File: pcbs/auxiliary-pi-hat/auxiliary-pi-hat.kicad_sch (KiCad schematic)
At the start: 18 parts, among them J1 Conn_01x02, J2 Raspberry Pi - Hat Template -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, J3 Conn_01x03, J4 Conn_01x03, J5 Conn_01x03, J6 Conn_01x03, J7 Conn_01x03, J8 Conn_01x04, J9 Conn_01x05, SW1 SW_Push, SW2 SW_Push, U1 YAAJ_WeAct_BlackPill_Part_Like

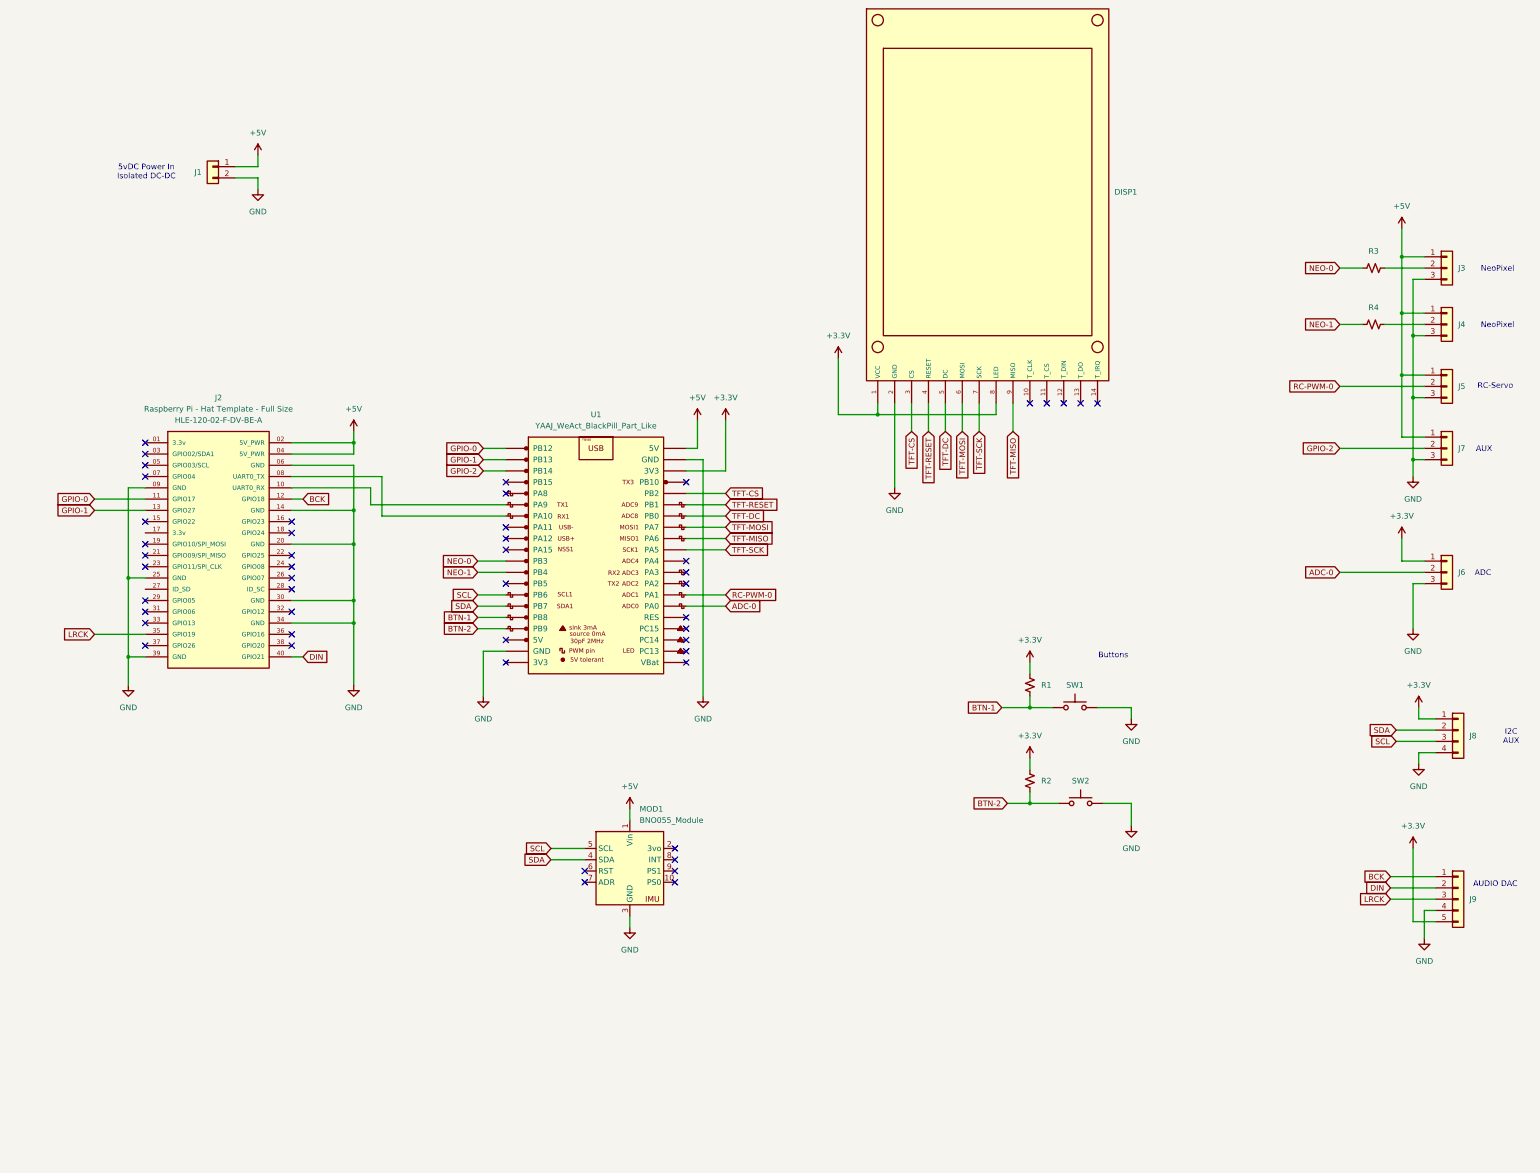
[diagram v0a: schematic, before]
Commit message: aux pcb update
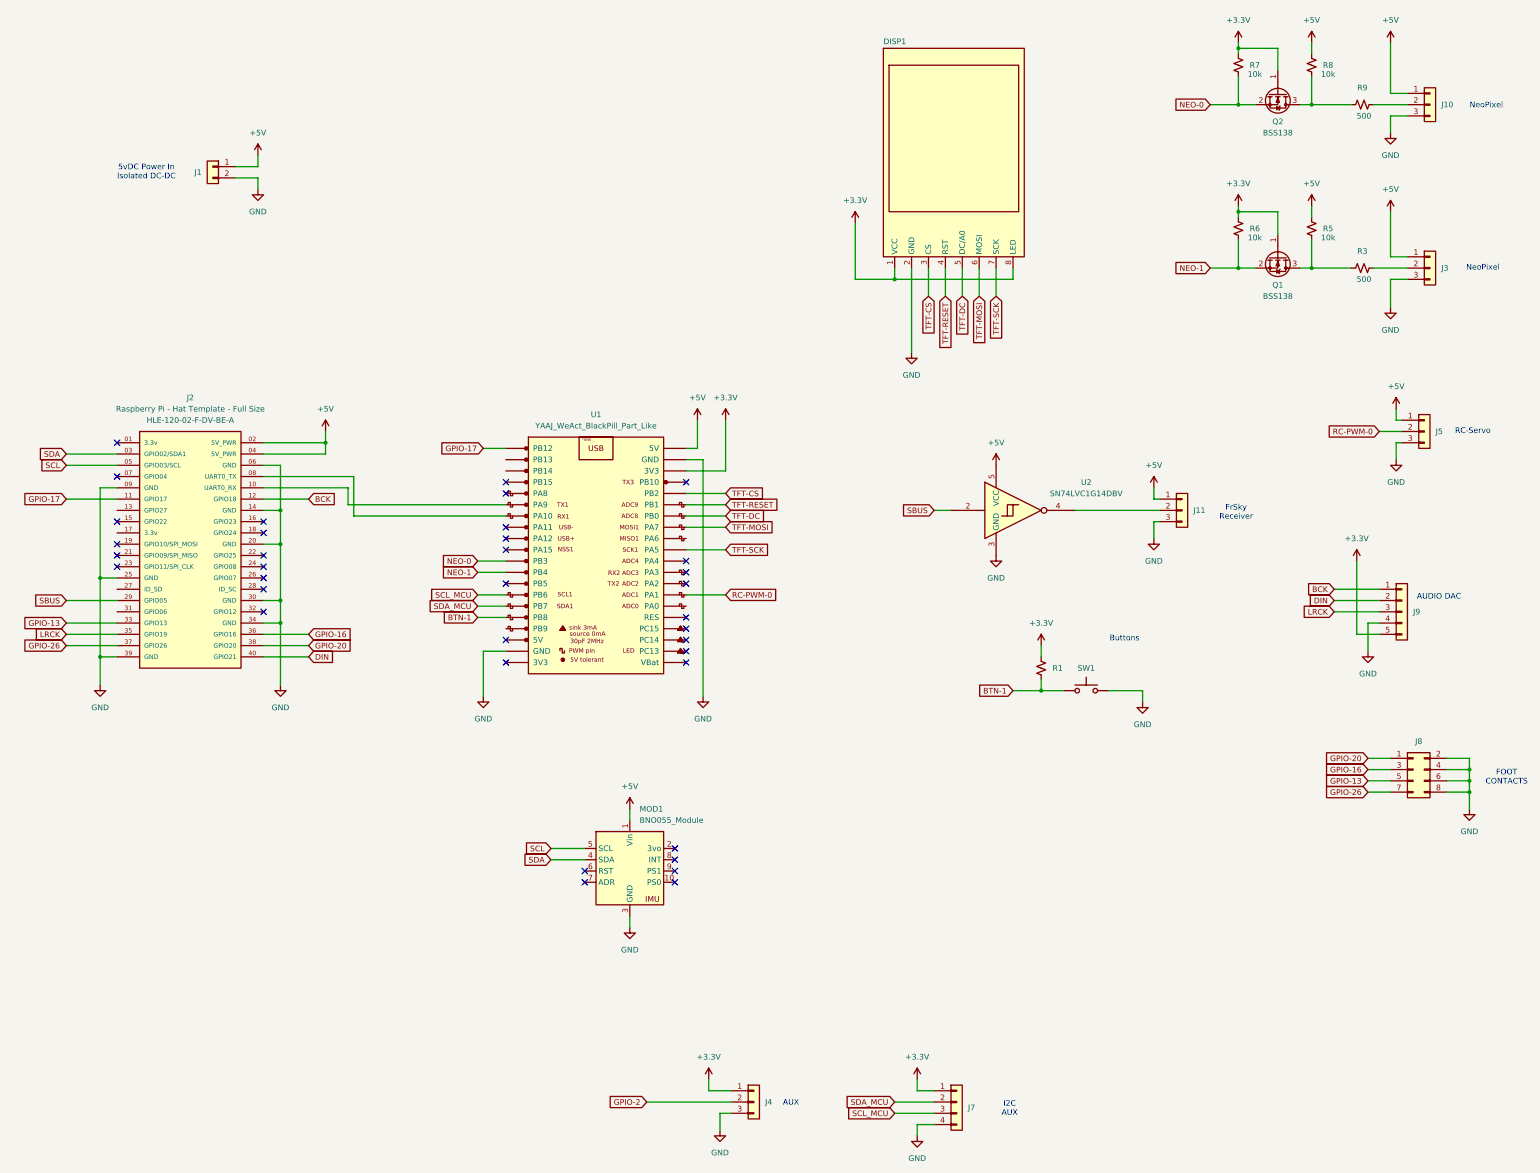
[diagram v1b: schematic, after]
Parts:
- removed DISP1: ~, displays:TFT LCD - 2.4 - 240x320, symbol displays:TFT_LCD_-_2.4_-_240x320
- removed J6, J7: Conn_01x03, Connector_JST:JST_ZH_B3B-ZR_1x03_P1.50mm_Vertical, symbol Connector_Generic:Conn_01x03
- removed J8: Conn_01x04, Connector_PinHeader_2.54mm:PinHeader_1x04_P2.54mm_Horizontal, symbol Connector_Generic:Conn_01x04
- removed R2, R4: R_Small_US, Resistor_SMD:R_1206_3216Metric, symbol Device:R_Small_US
- removed SW2: SW_Push, Button_Switch_THT:SW_PUSH_6mm_H4.3mm, symbol Switch:SW_Push
- added DISP1: ~, displays:LCD-Display-1.8-128x160-Hiletgo, symbol displays:LCD-Display-1.8-128x160-Hiletgo
- added J10, J11: Conn_01x03, Connector_JST:JST_ZH_B3B-ZR_1x03_P1.50mm_Vertical, symbol Connector_Generic:Conn_01x03
- added J7: Conn_01x04, Connector_JST:JST_ZH_B4B-ZR_1x04_P1.50mm_Vertical, symbol Connector_Generic:Conn_01x04
- added J8: Conn_02x04_Odd_Even, Connector_PinHeader_2.54mm:PinHeader_2x04_P2.54mm_Vertical, symbol Connector_Generic:Conn_02x04_Odd_Even
- added Q1, Q2: BSS138, Package_TO_SOT_SMD:SOT-23, symbol Transistor_FET:BSS138
- added R5, R6, R7, R8: 10k, Resistor_SMD:R_1206_3216Metric, symbol Device:R_Small_US
- added R9: 500, Resistor_SMD:R_1206_3216Metric, symbol Device:R_Small_US
- added U2: SN74LVC1G14DBV, Package_TO_SOT_SMD:SOT-23-5, symbol 74xGxx:SN74LVC1G14DBV
- J9: footprint Connector_PinHeader_2.54mm:PinHeader_1x05_P2.54mm_Horizontal -> Connector_JST:JST_ZH_B5B-ZR_1x05_P1.50mm_Vertical
- R3: value R_Small_US -> 500
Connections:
- net +3.3V: now also J4.1 (Pin_1), DISP1.1 (VCC), DISP1.8 (LED), J7.1 (Pin_1), Q1.1 (G), Q2.1 (G), R6.2, R7.2
- net +5V: now also J10.1 (Pin_1), J11.1 (Pin_1), R5.2, R8.2, U2.5 (VCC); no longer J4.1 (Pin_1)
- net GND: now also DISP1.2 (GND), J10.3 (Pin_3), J11.3 (Pin_3), J7.4 (Pin_4), J8.2 (Pin_2), J8.4 (Pin_4), J8.6 (Pin_6), J8.8 (Pin_8), U2.3 (GND)
- net GPIO-2: now also J4.2 (Pin_2); no longer U1.3 (PB14)
- net NEO-0: now also Q2.2 (S), R7.1; no longer R3.1
- net NEO-1: now also Q1.2 (S), R6.1
- net SCL: now also J2.05 (GPIO03/SCL); no longer U1.14 (PB6)
- net SDA: now also J2.03 (GPIO02/SDA1); no longer U1.15 (PB7)
- net TFT-CS: now also DISP1.3 (CS)
- net TFT-DC: now also DISP1.5 (DC/A0)
- net TFT-MOSI: now also DISP1.6 (MOSI)
- net TFT-RESET: now also DISP1.4 (RST)
- net TFT-SCK: now also DISP1.7 (SCK)
- net SBUS: now reaches J2.29 (GPIO05)
- net SBUS: now also U2.2
- net GPIO-13: now reaches J2.33 (GPIO13)
- net GPIO-13: now also J8.5 (Pin_5)
- net GPIO-16: now reaches J2.36 (GPIO16)
- net GPIO-16: now also J8.3 (Pin_3)
- net GPIO-26: now reaches J2.37 (GPIO26)
- net GPIO-26: now also J8.7 (Pin_7)
- net GPIO-20: now reaches J2.38 (GPIO20)
- net GPIO-20: now also J8.1 (Pin_1)
- net ADC-0: no longer names the net of U1.26 (PA0)
- net BTN-2: no longer names the net of U1.17 (PB9)
- net GPIO-0 renamed GPIO-17
- net GPIO-1: no longer names the net of J2.13 (GPIO27)
- net GPIO-1: no longer U1.2 (PB13)
- net TFT-MISO: no longer names the net of U1.32 (PA6)
- new net: J11.2 (Pin_2), U2.4
- new net: Q2.3 (D), R8.1, R9.1
- new net: J10.2 (Pin_2), R9.2
- new net: Q1.3 (D), R3.1, R5.1
- new net SCL_MCU: J7.3 (Pin_3), U1.14 (PB6)
- new net SDA_MCU: J7.2 (Pin_2), U1.15 (PB7)
- no-connect marks 49 -> 36
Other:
- note added: "FOOT CONTACTS"
- note added: "FrSky Receiver"
- note removed: "ADC"
- moved on the sheet: J2, J3, J5, J9, R1, R3, SW1
